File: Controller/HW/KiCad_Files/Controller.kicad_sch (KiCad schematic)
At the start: 8 parts, among them U5 AP1117-33

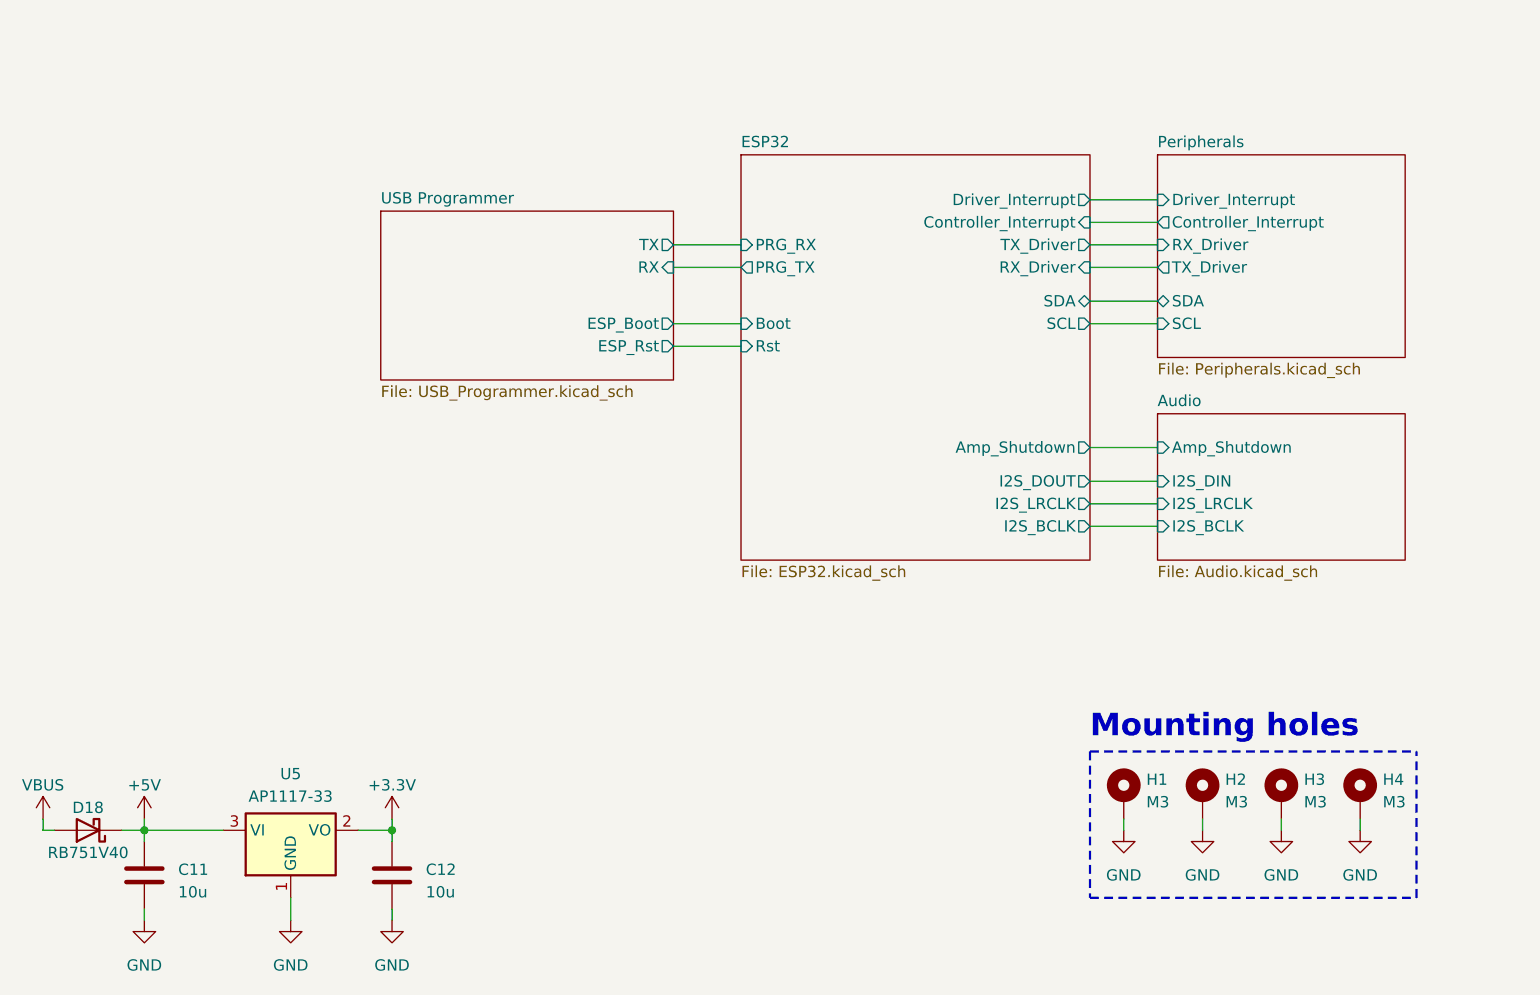
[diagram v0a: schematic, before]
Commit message: PCB Zwischenstand
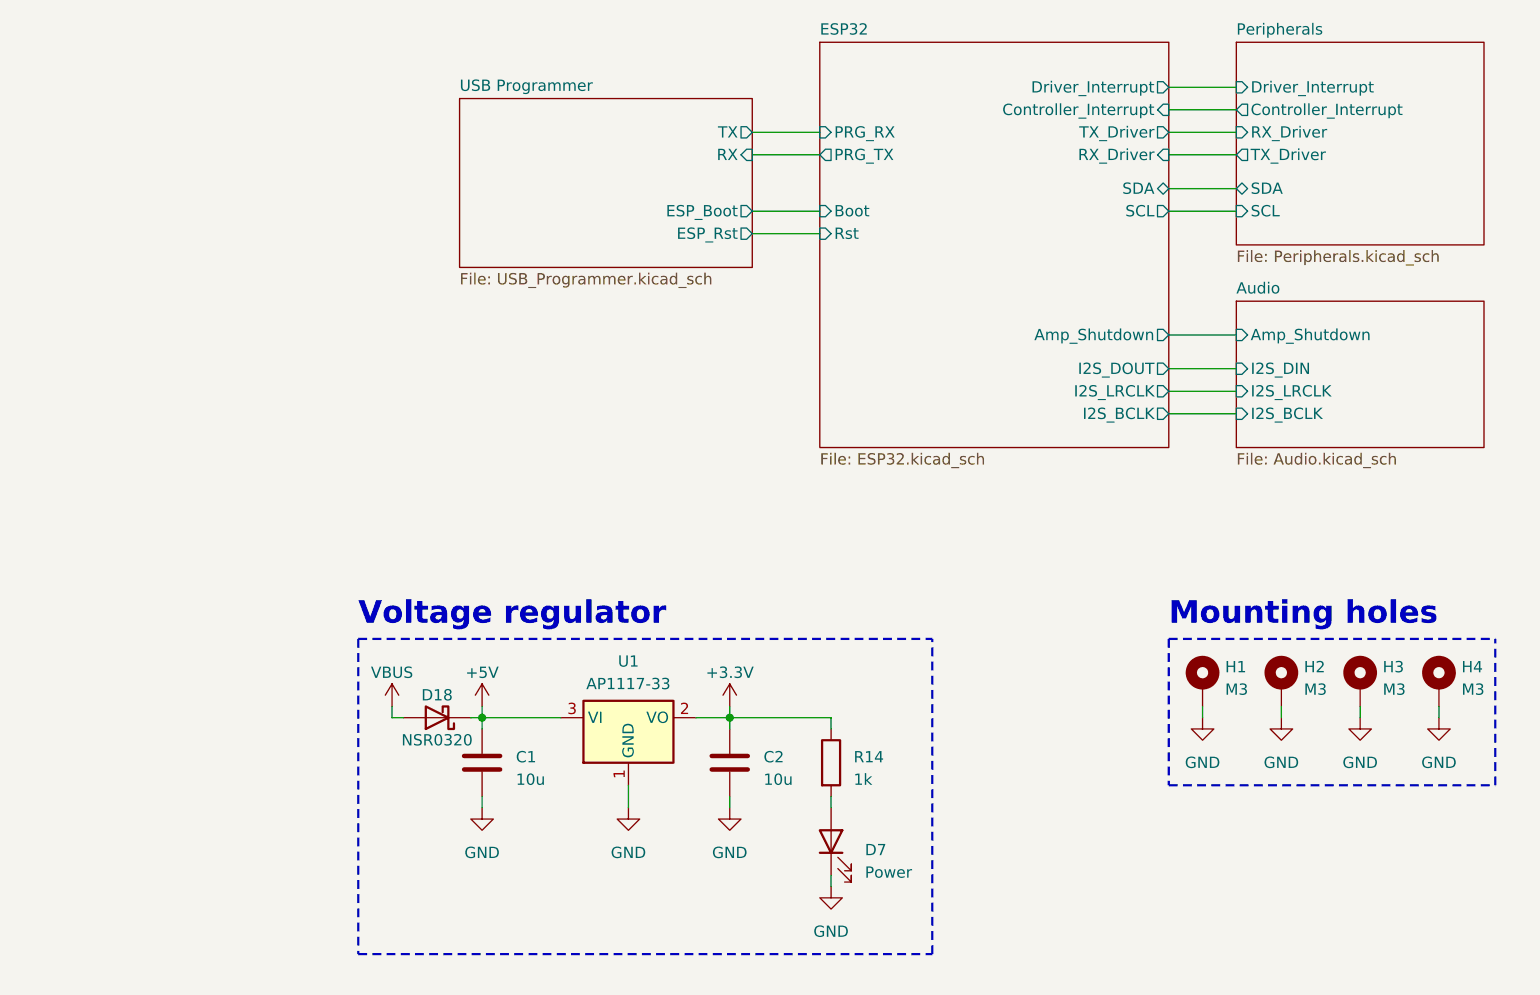
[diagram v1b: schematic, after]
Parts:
- added D7: Power, LED_SMD:LED_0805_2012Metric, symbol Device:LED
- added R14: 1k, Resistor_SMD:R_0805_2012Metric, symbol Device:R
- D18: value RB751V40 -> NSR0320; DigiKey 1727-6301-1-ND -> NSR0320MW2T3GOSCT-ND
- renumbered C11 to C1, C12 to C2, U5 to U1
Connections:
- net +3.3V: now also R14.1
- net GND: now also D7.1 (K)
- new net: D7.2 (A), R14.2
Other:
- note added: "Voltage regulator"
- moved on the sheet: C1, C2, D18, H1, H2, H3, H4, U1

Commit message: BOM update
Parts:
- C1, C2: DigiKey (none) -> 1276-1096-1-ND
- D7: DigiKey (none) -> 475-2488-1-ND
- R14: DigiKey (none) -> CR0805-FX-1001ELFCT-ND
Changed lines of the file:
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@@
+      (effects (font (size 1.27 1.27)) hide)
+    )
+    (property "DigiKey" "475-2488-1-ND" (at 130.81 148.59 0)
       (effects (font (size 1.27 1.27)) hide)
     )
@@
     )
     (property "Datasheet" "~" (at 119.38 139.7 0)
+      (effects (font (size 1.27 1.27)) hide)
+    )
+    (property "DigiKey" "1276-1096-1-ND" (at 119.38 139.7 0)
       (effects (font (size 1.27 1.27)) hide)
     )
@@
       (effects (font (size 1.27 1.27)) hide)
     )
+    (property "DigiKey" "1276-1096-1-ND" (at 91.44 139.7 0)
+      (effects (font (size 1.27 1.27)) hide)
+    )
     (pin "1")
     (pin "2")
@@
       (effects (font (size 1.27 1.27)) hide)
     )
+    (property "DigiKey" "CR0805-FX-1001ELFCT-ND" (at 130.81 139.7 0)
+      (effects (font (size 1.27 1.27)) hide)
+    )
